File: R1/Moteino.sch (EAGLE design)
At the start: 20 parts, among them IC3 MCP1703CB, X1 16 MHz

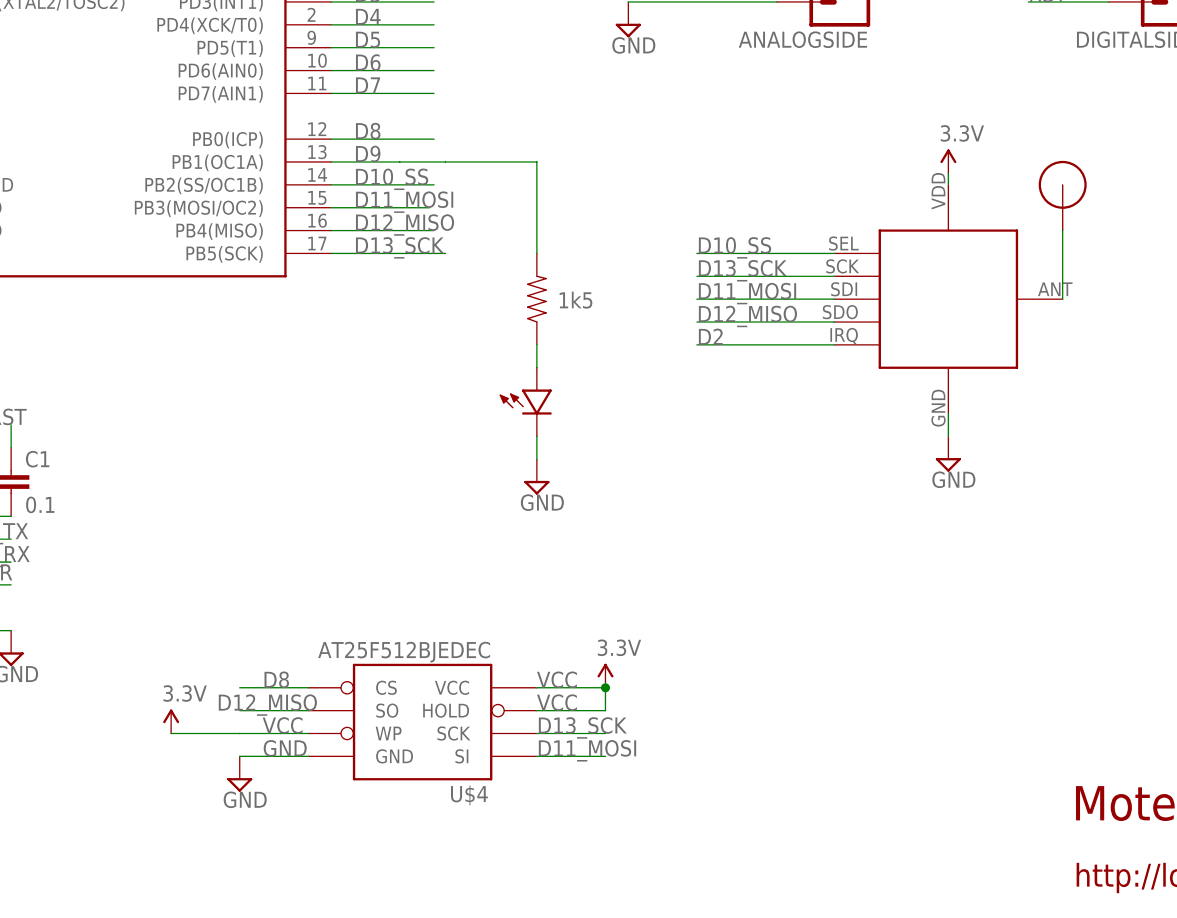
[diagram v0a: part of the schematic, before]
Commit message: R2 Update
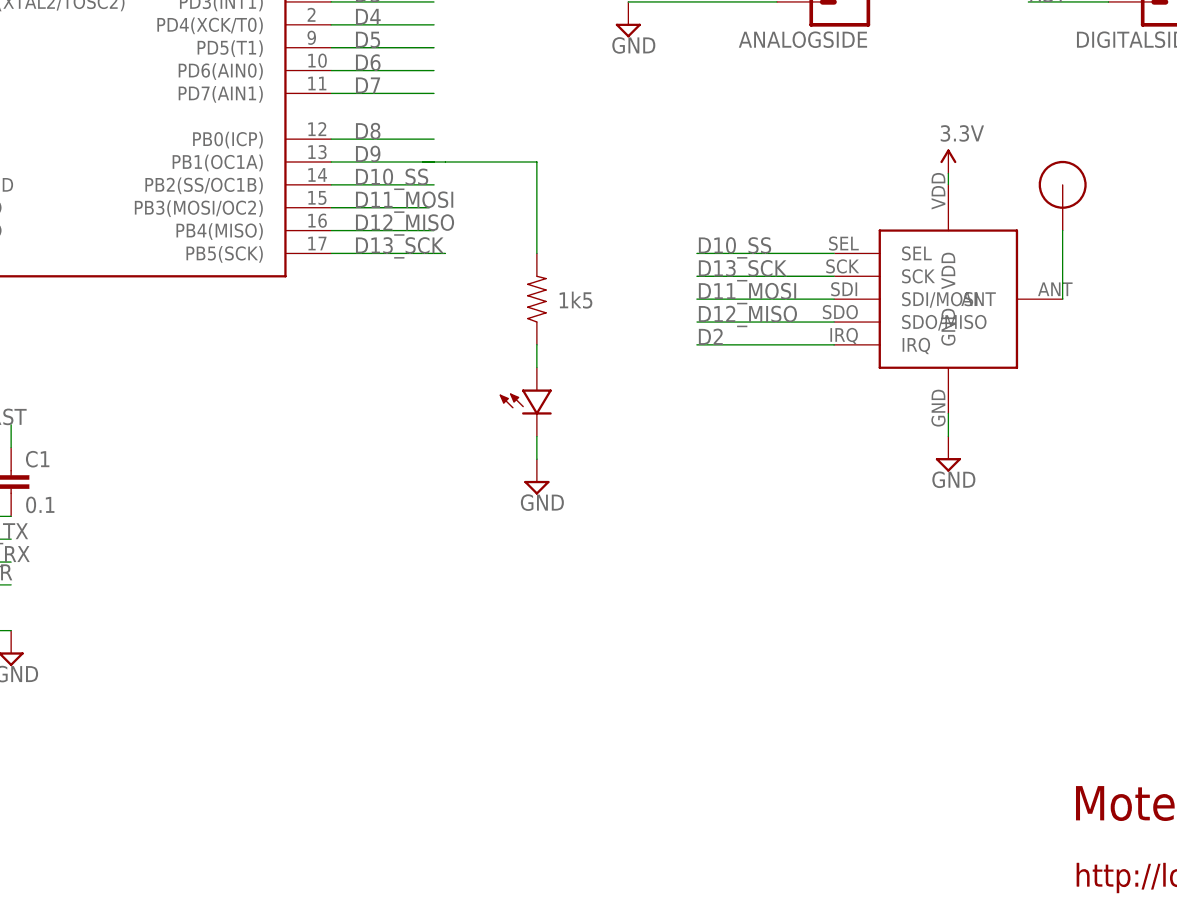
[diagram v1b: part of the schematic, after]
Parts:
- removed U$4: AT25F512BJEDEC, LowPowerLab:AT25F512BJEDEC
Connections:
- net D11_MOSI: no longer U$4.SI
- net D12_MISO: no longer U$4.SO
- net D13_SCK: no longer U$4.SCK
- net D8: no longer U$4.CS
- net GND: no longer U$4.GND
- net VCC: no longer U$4.HOLD, U$4.VCC, U$4.WP
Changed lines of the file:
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@@
 <part name="RFM12B" library="LowPowerLab" deviceset="RFM12B_MINPADS" device=""/>
 <part name="U$1" library="LowPowerLab" deviceset="RFM12B_ANTENNA" device=""/>
-<part name="U$4" library="LowPowerLab" deviceset="AT25F512B" device="JEDEC"/>
-<part name="SUPPLY8" library="supply2" deviceset="GND" device=""/>
-<part name="P+4" library="SparkFun" deviceset="VCC" device="" value="3.3V"/>
-<part name="P+5" library="SparkFun" deviceset="VCC" device="" value="3.3V"/>
 </parts>
 <sheets>
@@
 <instance part="RFM12B" gate="G$1" x="152.4" y="73.66" smashed="yes"/>
 <instance part="U$1" gate="G$1" x="165.1" y="86.36" rot="R90"/>
-<instance part="U$4" gate="G$1" x="93.98" y="27.94"/>
-<instance part="SUPPLY8" gate="GND" x="73.66" y="20.32"/>
-<instance part="P+4" gate="1" x="114.3" y="30.48"/>
-<instance part="P+5" gate="1" x="66.04" y="25.4"/>
 </instances>
 <busses>
@@
 <wire x1="106.68" y1="55.88" x2="106.68" y2="58.42" width="0.1524" layer="91"/>
 </segment>
-<segment>
-<wire x1="81.28" y1="22.86" x2="73.66" y2="22.86" width="0.1524" layer="91"/>
-<pinref part="U$4" gate="G$1" pin="GND"/>
-<label x="76.2" y="22.86" size="1.778" layer="95"/>
-<pinref part="SUPPLY8" gate="GND" pin="GND"/>
-</segment>
 </net>
 <net name="D10_SS" class="0">
@@
 <pinref part="P+3" gate="1" pin="VCC"/>
 </segment>
-<segment>
-<wire x1="106.68" y1="30.48" x2="114.3" y2="30.48" width="0.1524" layer="91"/>
-<pinref part="U$4" gate="G$1" pin="VCC"/>
-<label x="106.68" y="30.48" size="1.778" layer="95"/>
-<pinref part="P+4" gate="1" pin="VCC"/>
-<wire x1="106.68" y1="27.94" x2="114.3" y2="27.94" width="0.1524" layer="91"/>
-<pinref part="U$4" gate="G$1" pin="HOLD"/>
-<label x="106.68" y="27.94" size="1.778" layer="95"/>
-<wire x1="114.3" y1="27.94" x2="114.3" y2="30.48" width="0.1524" layer="91"/>
-<junction x="114.3" y="30.48"/>
-</segment>
-<segment>
-<wire x1="81.28" y1="25.4" x2="73.66" y2="25.4" width="0.1524" layer="91"/>
-<pinref part="U$4" gate="G$1" pin="WP"/>
-<label x="76.2" y="25.4" size="1.778" layer="95"/>
-<pinref part="P+5" gate="1" pin="VCC"/>
-<wire x1="73.66" y1="25.4" x2="66.04" y2="25.4" width="0.1524" layer="91"/>
-</segment>
 </net>
 <net name="D9" class="0">
 <segment>
-<wire x1="83.82" y1="88.9" x2="91.44" y2="88.9" width="0.1524" layer="91"/>
+<wire x1="83.82" y1="88.9" x2="93.98" y2="88.9" width="0.1524" layer="91"/>
 <label x="86.36" y="88.9" size="1.778" layer="95"/>
 <pinref part="ATMEGA328" gate="G$1" pin="PB1(OC1A)"/>
 <pinref part="R2" gate="G$1" pin="2"/>
+<wire x1="93.98" y1="88.9" x2="95.25" y2="88.9" width="0.1524" layer="91"/>
 <wire x1="96.52" y1="88.9" x2="106.68" y2="88.9" width="0.1524" layer="91"/>
 <wire x1="106.68" y1="88.9" x2="106.68" y2="78.74" width="0.1524" layer="91"/>
-<wire x1="96.52" y1="88.9" x2="91.44" y2="88.9" width="0.1524" layer="91"/>
+<wire x1="96.52" y1="88.9" x2="93.98" y2="88.9" width="0.1524" layer="91"/>
 </segment>
 <segment>
@@
 <label x="161.29" y="124.46" size="1.778" layer="95"/>
 </segment>
-<segment>
-<wire x1="81.28" y1="30.48" x2="73.66" y2="30.48" width="0.1524" layer="91"/>
-<pinref part="U$4" gate="G$1" pin="CS"/>
-<label x="76.2" y="30.48" size="1.778" layer="95"/>
-</segment>
 </net>
 <net name="D7" class="0">
@@
 <label x="86.36" y="83.82" size="1.778" layer="95"/>
 </segment>
-<segment>
-<wire x1="106.68" y1="22.86" x2="114.3" y2="22.86" width="0.1524" layer="91"/>
-<pinref part="U$4" gate="G$1" pin="SI"/>
-<label x="106.68" y="22.86" size="1.778" layer="95"/>
-</segment>
 </net>
 <net name="D12_MISO" class="0">
@@
 <pinref part="RFM12B" gate="G$1" pin="SDO/MISO"/>
 </segment>
-<segment>
-<wire x1="81.28" y1="27.94" x2="73.66" y2="27.94" width="0.1524" layer="91"/>
-<pinref part="U$4" gate="G$1" pin="SO"/>
-<label x="71.12" y="27.94" size="1.778" layer="95"/>
-</segment>
 </net>
 <net name="D13_SCK" class="0">
@@
 <pinref part="RFM12B" gate="G$1" pin="SCK"/>
 </segment>
-<segment>
-<wire x1="106.68" y1="25.4" x2="114.3" y2="25.4" width="0.1524" layer="91"/>
-<pinref part="U$4" gate="G$1" pin="SCK"/>
-<label x="106.68" y="25.4" size="1.778" layer="95"/>
-</segment>
-</net>
+</net>
